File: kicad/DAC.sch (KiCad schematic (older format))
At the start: 27 parts, among them Q1 Q_DUAL_NMOS_S1G1D2S2G2D1, U6 TCR2EE48, U7 DS3911, U8 TSV994IPT

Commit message: 0603 most passives
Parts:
- R11, R12, R13, R14, R15, R16, R17, R18, R19, R20: footprint Resistor_SMD:R_0805_2012Metric_Pad1.20x1.40mm_HandSolder -> Resistor_SMD:R_0603_1608Metric_Pad0.98x0.95mm_HandSolder
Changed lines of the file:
@@
 F 0 "R13" V 8250 3100 50  0000 L CNN
 F 1 "1k" V 8350 3100 50  0000 L CNN
-F 2 "Resistor_SMD:R_0805_2012Metric_Pad1.20x1.40mm_HandSolder" V 8280 3150 50  0001 C CNN
+F 2 "Resistor_SMD:R_0603_1608Metric_Pad0.98x0.95mm_HandSolder" V 8280 3150 50  0001 C CNN
 F 3 "~" H 8350 3150 50  0001 C CNN
 	1    8350 3150
@@
 F 0 "R17" V 8550 3100 50  0000 L CNN
 F 1 "1k" V 8650 3100 50  0000 L CNN
-F 2 "Resistor_SMD:R_0805_2012Metric_Pad1.20x1.40mm_HandSolder" V 8580 3150 50  0001 C CNN
+F 2 "Resistor_SMD:R_0603_1608Metric_Pad0.98x0.95mm_HandSolder" V 8580 3150 50  0001 C CNN
 F 3 "~" H 8650 3150 50  0001 C CNN
 	1    8650 3150
@@
 F 0 "R14" V 8250 3550 50  0000 L CNN
 F 1 "1k" V 8350 3550 50  0000 L CNN
-F 2 "Resistor_SMD:R_0805_2012Metric_Pad1.20x1.40mm_HandSolder" V 8280 3600 50  0001 C CNN
+F 2 "Resistor_SMD:R_0603_1608Metric_Pad0.98x0.95mm_HandSolder" V 8280 3600 50  0001 C CNN
 F 3 "~" H 8350 3600 50  0001 C CNN
 	1    8350 3600
@@
 F 0 "R18" V 8550 3550 50  0000 L CNN
 F 1 "1k" V 8650 3550 50  0000 L CNN
-F 2 "Resistor_SMD:R_0805_2012Metric_Pad1.20x1.40mm_HandSolder" V 8580 3600 50  0001 C CNN
+F 2 "Resistor_SMD:R_0603_1608Metric_Pad0.98x0.95mm_HandSolder" V 8580 3600 50  0001 C CNN
 F 3 "~" H 8650 3600 50  0001 C CNN
 	1    8650 3600
@@
 F 0 "R15" V 8250 4050 50  0000 L CNN
 F 1 "1k" V 8350 4050 50  0000 L CNN
-F 2 "Resistor_SMD:R_0805_2012Metric_Pad1.20x1.40mm_HandSolder" V 8280 4100 50  0001 C CNN
+F 2 "Resistor_SMD:R_0603_1608Metric_Pad0.98x0.95mm_HandSolder" V 8280 4100 50  0001 C CNN
 F 3 "~" H 8350 4100 50  0001 C CNN
 	1    8350 4100
@@
 F 0 "R19" V 8550 4050 50  0000 L CNN
 F 1 "1k" V 8650 4050 50  0000 L CNN
-F 2 "Resistor_SMD:R_0805_2012Metric_Pad1.20x1.40mm_HandSolder" V 8580 4100 50  0001 C CNN
+F 2 "Resistor_SMD:R_0603_1608Metric_Pad0.98x0.95mm_HandSolder" V 8580 4100 50  0001 C CNN
 F 3 "~" H 8650 4100 50  0001 C CNN
 	1    8650 4100
@@
 F 0 "R16" V 8250 4550 50  0000 L CNN
 F 1 "1k" V 8350 4550 50  0000 L CNN
-F 2 "Resistor_SMD:R_0805_2012Metric_Pad1.20x1.40mm_HandSolder" V 8280 4600 50  0001 C CNN
+F 2 "Resistor_SMD:R_0603_1608Metric_Pad0.98x0.95mm_HandSolder" V 8280 4600 50  0001 C CNN
 F 3 "~" H 8350 4600 50  0001 C CNN
 	1    8350 4600
@@
 F 0 "R20" V 8550 4550 50  0000 L CNN
 F 1 "1k" V 8650 4550 50  0000 L CNN
-F 2 "Resistor_SMD:R_0805_2012Metric_Pad1.20x1.40mm_HandSolder" V 8580 4600 50  0001 C CNN
+F 2 "Resistor_SMD:R_0603_1608Metric_Pad0.98x0.95mm_HandSolder" V 8580 4600 50  0001 C CNN
 F 3 "~" H 8650 4600 50  0001 C CNN
 	1    8650 4600
@@
 F 0 "R11" H 4170 5396 50  0000 L CNN
 F 1 "4.7k" H 4170 5305 50  0000 L CNN
-F 2 "Resistor_SMD:R_0805_2012Metric_Pad1.20x1.40mm_HandSolder" V 4030 5350 50  0001 C CNN
+F 2 "Resistor_SMD:R_0603_1608Metric_Pad0.98x0.95mm_HandSolder" V 4030 5350 50  0001 C CNN
 F 3 "~" H 4100 5350 50  0001 C CNN
 	1    4100 5350
@@
 F 0 "R12" H 4470 5396 50  0000 L CNN
 F 1 "4.7k" H 4470 5305 50  0000 L CNN
-F 2 "Resistor_SMD:R_0805_2012Metric_Pad1.20x1.40mm_HandSolder" V 4330 5350 50  0001 C CNN
+F 2 "Resistor_SMD:R_0603_1608Metric_Pad0.98x0.95mm_HandSolder" V 4330 5350 50  0001 C CNN
 F 3 "~" H 4400 5350 50  0001 C CNN
 	1    4400 5350

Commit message: adding jlc fields
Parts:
- C12, C14, C15, C16, C17, C18, C19, C20, C21, C22, C23: JLC (none) -> 0603; LCSC (none) -> C30926
- C13, C24: JLC (none) -> 0805; LCSC (none) -> C215803
- U6: JLC (none) -> SOT-23-5; LCSC (none) -> C698019
- U7: JLC (none) -> TDFN-14-EP(3x3); LCSC (none) -> C1554592
- U8: JLC (none) -> TSSOP-14; LCSC (none) -> C503311
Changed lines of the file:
@@
 F 2 "quadrant:SON40P300X500X80-15N" H 7900 3600 50  0001 C CNN
 F 3 "" H 7900 3600 50  0001 C CNN
+F 4 "TDFN-14-EP(3x3)" H 7900 3600 50  0001 C CNN "JLC"
+F 5 "C1554592" H 7900 3600 50  0001 C CNN "LCSC"
 	1    7900 3600
 	1    0    0    -1
@@
 F 2 "Capacitor_SMD:C_0603_1608Metric_Pad1.08x0.95mm_HandSolder" H 7150 3200 50  0001 C CNN
 F 3 "~" H 7150 3200 50  0001 C CNN
+F 4 "0603" H 7150 3200 50  0001 C CNN "JLC"
+F 5 "C30926" H 7150 3200 50  0001 C CNN "LCSC"
 	1    7150 3200
 	1    0    0    -1
@@
 F 2 "Capacitor_SMD:C_0603_1608Metric_Pad1.08x0.95mm_HandSolder" H 7150 3600 50  0001 C CNN
 F 3 "~" H 7150 3600 50  0001 C CNN
+F 4 "0603" H 7150 3600 50  0001 C CNN "JLC"
+F 5 "C30926" H 7150 3600 50  0001 C CNN "LCSC"
 	1    7150 3600
 	1    0    0    -1
@@
 F 2 "Capacitor_SMD:C_0603_1608Metric_Pad1.08x0.95mm_HandSolder" H 8500 3250 50  0001 C CNN
 F 3 "~" H 8500 3250 50  0001 C CNN
+F 4 "0603" H 8500 3250 50  0001 C CNN "JLC"
+F 5 "C30926" H 8500 3250 50  0001 C CNN "LCSC"
 	1    8500 3250
 	-1   0    0    1
@@
 F 2 "Capacitor_SMD:C_0603_1608Metric_Pad1.08x0.95mm_HandSolder" H 8800 3250 50  0001 C CNN
 F 3 "~" H 8800 3250 50  0001 C CNN
+F 4 "0603" H 8800 3250 50  0001 C CNN "JLC"
+F 5 "C30926" H 8800 3250 50  0001 C CNN "LCSC"
 	1    8800 3250
 	-1   0    0    1
@@
 F 2 "Capacitor_SMD:C_0603_1608Metric_Pad1.08x0.95mm_HandSolder" H 8500 3700 50  0001 C CNN
 F 3 "~" H 8500 3700 50  0001 C CNN
+F 4 "0603" H 8500 3700 50  0001 C CNN "JLC"
+F 5 "C30926" H 8500 3700 50  0001 C CNN "LCSC"
 	1    8500 3700
 	-1   0    0    1
@@
 F 2 "Capacitor_SMD:C_0603_1608Metric_Pad1.08x0.95mm_HandSolder" H 8800 3700 50  0001 C CNN
 F 3 "~" H 8800 3700 50  0001 C CNN
+F 4 "0603" H 8800 3700 50  0001 C CNN "JLC"
+F 5 "C30926" H 8800 3700 50  0001 C CNN "LCSC"
 	1    8800 3700
 	-1   0    0    1
@@
 F 2 "Capacitor_SMD:C_0603_1608Metric_Pad1.08x0.95mm_HandSolder" H 8500 4200 50  0001 C CNN
 F 3 "~" H 8500 4200 50  0001 C CNN
+F 4 "0603" H 8500 4200 50  0001 C CNN "JLC"
+F 5 "C30926" H 8500 4200 50  0001 C CNN "LCSC"
 	1    8500 4200
 	-1   0    0    1
@@
 F 2 "Capacitor_SMD:C_0603_1608Metric_Pad1.08x0.95mm_HandSolder" H 8800 4200 50  0001 C CNN
 F 3 "~" H 8800 4200 50  0001 C CNN
+F 4 "0603" H 8800 4200 50  0001 C CNN "JLC"
+F 5 "C30926" H 8800 4200 50  0001 C CNN "LCSC"
 	1    8800 4200
 	-1   0    0    1
@@
 F 2 "Capacitor_SMD:C_0603_1608Metric_Pad1.08x0.95mm_HandSolder" H 8800 4700 50  0001 C CNN
 F 3 "~" H 8800 4700 50  0001 C CNN
+F 4 "0603" H 8800 4700 50  0001 C CNN "JLC"
+F 5 "C30926" H 8800 4700 50  0001 C CNN "LCSC"
 	1    8800 4700
 	-1   0    0    1
@@
 F 2 "Package_SO:TSSOP-14_4.4x5mm_P0.65mm" H 9450 4200 50  0001 C CNN
 F 3 "~" H 9450 4200 50  0001 C CNN
+F 4 "TSSOP-14" H 9450 4200 50  0001 C CNN "JLC"
+F 5 "C503311" H 9450 4200 50  0001 C CNN "LCSC"
 	1    9450 4200
 	1    0    0    -1
@@
 F 2 "Package_SO:TSSOP-14_4.4x5mm_P0.65mm" H 9450 4700 50  0001 C CNN
 F 3 "~" H 9450 4700 50  0001 C CNN
+F 4 "TSSOP-14" H 9450 4700 50  0001 C CNN "JLC"
+F 5 "C503311" H 9450 4700 50  0001 C CNN "LCSC"
 	2    9450 4700
 	1    0    0    -1
@@
 F 2 "Package_SO:TSSOP-14_4.4x5mm_P0.65mm" H 9450 3700 50  0001 C CNN
 F 3 "~" H 9450 3700 50  0001 C CNN
+F 4 "TSSOP-14" H 9450 3700 50  0001 C CNN "JLC"
+F 5 "C503311" H 9450 3700 50  0001 C CNN "LCSC"
 	3    9450 3700
 	1    0    0    -1
@@
 F 2 "Package_SO:TSSOP-14_4.4x5mm_P0.65mm" H 9450 3250 50  0001 C CNN
 F 3 "~" H 9450 3250 50  0001 C CNN
+F 4 "TSSOP-14" H 9450 3250 50  0001 C CNN "JLC"
+F 5 "C503311" H 9450 3250 50  0001 C CNN "LCSC"
 	4    9450 3250
 	1    0    0    -1
@@
 F 2 "Package_SO:TSSOP-14_4.4x5mm_P0.65mm" H 9750 5350 50  0001 C CNN
 F 3 "~" H 9750 5350 50  0001 C CNN
+F 4 "TSSOP-14" H 9750 5350 50  0001 C CNN "JLC"
+F 5 "C503311" H 9750 5350 50  0001 C CNN "LCSC"
 	5    9750 5350
 	1    0    0    -1
@@
 F 2 "Capacitor_SMD:C_0805_2012Metric_Pad1.18x1.45mm_HandSolder" H 9388 5200 50  0001 C CNN
 F 3 "~" H 9350 5350 50  0001 C CNN
+F 4 "0805" H 9350 5350 50  0001 C CNN "JLC"
+F 5 "C215803" H 9350 5350 50  0001 C CNN "LCSC"
 	1    9350 5350
 	1    0    0    -1
@@
 F 3 "" H 4550 3550 50  0001 C CNN
 F 4 "https://www.digikey.com/en/products/detail/toshiba-semiconductor-and-storage/TCR2EE48-LM/5114341" H 4550 3550 50  0001 C CNN "digikey"
+F 5 "SOT-23-5" H 4550 3550 50  0001 C CNN "JLC"
+F 6 "C698019" H 4550 3550 50  0001 C CNN "LCSC"
 	1    4550 3550
 	1    0    0    -1
@@
 F 2 "Capacitor_SMD:C_0603_1608Metric_Pad1.08x0.95mm_HandSolder" H 3900 3600 50  0001 C CNN
 F 3 "~" H 3900 3600 50  0001 C CNN
+F 4 "0603" H 3900 3600 50  0001 C CNN "JLC"
+F 5 "C30926" H 3900 3600 50  0001 C CNN "LCSC"
 	1    3900 3600
 	1    0    0    -1
@@
 F 2 "Capacitor_SMD:C_0805_2012Metric_Pad1.18x1.45mm_HandSolder" H 5100 3600 50  0001 C CNN
 F 3 "~" H 5100 3600 50  0001 C CNN
+F 4 "0805" H 5100 3600 50  0001 C CNN "JLC"
+F 5 "C215803" H 5100 3600 50  0001 C CNN "LCSC"
 	1    5100 3600
 	1    0    0    -1
@@
 F 2 "Capacitor_SMD:C_0603_1608Metric_Pad1.08x0.95mm_HandSolder" H 8500 4700 50  0001 C CNN
 F 3 "~" H 8500 4700 50  0001 C CNN
+F 4 "0603" H 8500 4700 50  0001 C CNN "JLC"
+F 5 "C30926" H 8500 4700 50  0001 C CNN "LCSC"
 	1    8500 4700
 	-1   0    0    1

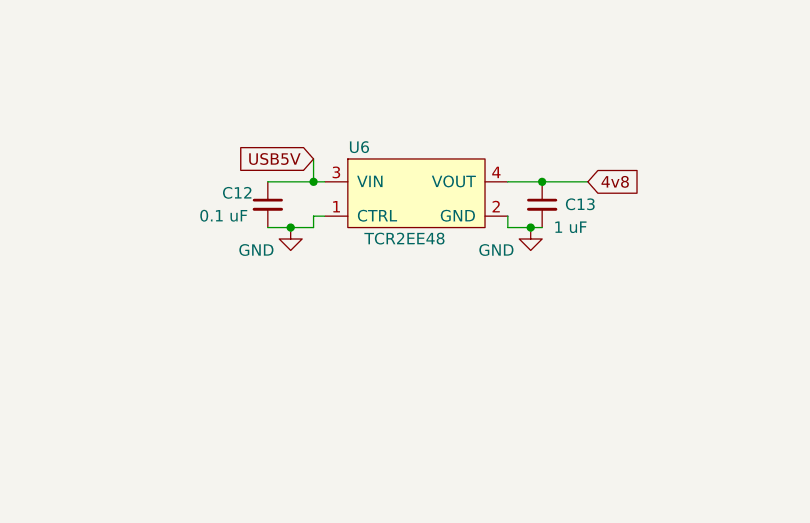
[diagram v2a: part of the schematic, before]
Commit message: more jlc fields
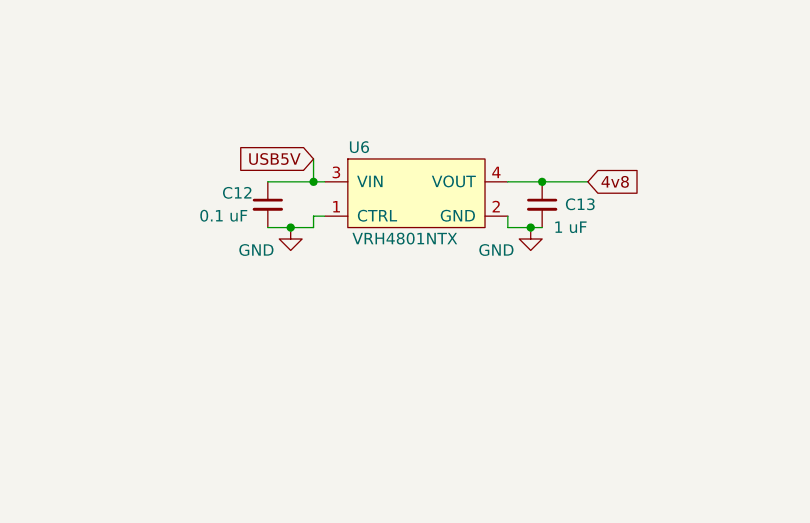
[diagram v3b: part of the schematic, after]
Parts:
- C12, C13, C14, C15, C16, C17, C18, C19, C20, C21, C22, C23, C24, U7, U8: ordered (none) -> y
- R11, R12: JLC (none) -> 0603; LCSC (none) -> C23162; ordered (none) -> y
- R13, R14, R15, R16, R17, R18, R19, R20: JLC (none) -> 0603; LCSC (none) -> C21190; ordered (none) -> y
- U6: value TCR2EE48 -> VRH4801NTX; ordered (none) -> ---
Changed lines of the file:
@@
 F 4 "TDFN-14-EP(3x3)" H 7900 3600 50  0001 C CNN "JLC"
 F 5 "C1554592" H 7900 3600 50  0001 C CNN "LCSC"
+F 6 "y" H 7900 3600 50  0001 C CNN "ordered"
 	1    7900 3600
 	1    0    0    -1
@@
 F 4 "0603" H 7150 3200 50  0001 C CNN "JLC"
 F 5 "C30926" H 7150 3200 50  0001 C CNN "LCSC"
+F 6 "y" H 7150 3200 50  0001 C CNN "ordered"
 	1    7150 3200
 	1    0    0    -1
@@
 F 4 "0603" H 7150 3600 50  0001 C CNN "JLC"
 F 5 "C30926" H 7150 3600 50  0001 C CNN "LCSC"
+F 6 "y" H 7150 3600 50  0001 C CNN "ordered"
 	1    7150 3600
 	1    0    0    -1
@@
 F 2 "Resistor_SMD:R_0603_1608Metric_Pad0.98x0.95mm_HandSolder" V 8280 3150 50  0001 C CNN
 F 3 "~" H 8350 3150 50  0001 C CNN
+F 4 "0603" H 8350 3150 50  0001 C CNN "JLC"
+F 5 " C21190 " H 8350 3150 50  0001 C CNN "LCSC"
+F 6 "y" H 8350 3150 50  0001 C CNN "ordered"
 	1    8350 3150
 	0    -1   1    0
@@
 F 4 "0603" H 8500 3250 50  0001 C CNN "JLC"
 F 5 "C30926" H 8500 3250 50  0001 C CNN "LCSC"
+F 6 "y" H 8500 3250 50  0001 C CNN "ordered"
 	1    8500 3250
 	-1   0    0    1
@@
 F 4 "0603" H 8800 3250 50  0001 C CNN "JLC"
 F 5 "C30926" H 8800 3250 50  0001 C CNN "LCSC"
+F 6 "y" H 8800 3250 50  0001 C CNN "ordered"
 	1    8800 3250
 	-1   0    0    1
@@
 F 2 "Resistor_SMD:R_0603_1608Metric_Pad0.98x0.95mm_HandSolder" V 8580 3150 50  0001 C CNN
 F 3 "~" H 8650 3150 50  0001 C CNN
+F 4 "0603" H 8650 3150 50  0001 C CNN "JLC"
+F 5 " C21190 " H 8650 3150 50  0001 C CNN "LCSC"
+F 6 "y" H 8650 3150 50  0001 C CNN "ordered"
 	1    8650 3150
 	0    -1   1    0
@@
 F 2 "Resistor_SMD:R_0603_1608Metric_Pad0.98x0.95mm_HandSolder" V 8280 3600 50  0001 C CNN
 F 3 "~" H 8350 3600 50  0001 C CNN
+F 4 "0603" H 8350 3600 50  0001 C CNN "JLC"
+F 5 " C21190 " H 8350 3600 50  0001 C CNN "LCSC"
+F 6 "y" H 8350 3600 50  0001 C CNN "ordered"
 	1    8350 3600
 	0    -1   1    0
@@
 F 4 "0603" H 8500 3700 50  0001 C CNN "JLC"
 F 5 "C30926" H 8500 3700 50  0001 C CNN "LCSC"
+F 6 "y" H 8500 3700 50  0001 C CNN "ordered"
 	1    8500 3700
 	-1   0    0    1
@@
 F 4 "0603" H 8800 3700 50  0001 C CNN "JLC"
 F 5 "C30926" H 8800 3700 50  0001 C CNN "LCSC"
+F 6 "y" H 8800 3700 50  0001 C CNN "ordered"
 	1    8800 3700
 	-1   0    0    1
@@
 F 2 "Resistor_SMD:R_0603_1608Metric_Pad0.98x0.95mm_HandSolder" V 8580 3600 50  0001 C CNN
 F 3 "~" H 8650 3600 50  0001 C CNN
+F 4 "0603" H 8650 3600 50  0001 C CNN "JLC"
+F 5 " C21190 " H 8650 3600 50  0001 C CNN "LCSC"
+F 6 "y" H 8650 3600 50  0001 C CNN "ordered"
 	1    8650 3600
 	0    -1   1    0
@@
 F 2 "Resistor_SMD:R_0603_1608Metric_Pad0.98x0.95mm_HandSolder" V 8280 4100 50  0001 C CNN
 F 3 "~" H 8350 4100 50  0001 C CNN
+F 4 "0603" H 8350 4100 50  0001 C CNN "JLC"
+F 5 " C21190 " H 8350 4100 50  0001 C CNN "LCSC"
+F 6 "y" H 8350 4100 50  0001 C CNN "ordered"
 	1    8350 4100
 	0    -1   1    0
@@
 F 4 "0603" H 8500 4200 50  0001 C CNN "JLC"
 F 5 "C30926" H 8500 4200 50  0001 C CNN "LCSC"
+F 6 "y" H 8500 4200 50  0001 C CNN "ordered"
 	1    8500 4200
 	-1   0    0    1
@@
 F 4 "0603" H 8800 4200 50  0001 C CNN "JLC"
 F 5 "C30926" H 8800 4200 50  0001 C CNN "LCSC"
+F 6 "y" H 8800 4200 50  0001 C CNN "ordered"
 	1    8800 4200
 	-1   0    0    1
@@
 F 2 "Resistor_SMD:R_0603_1608Metric_Pad0.98x0.95mm_HandSolder" V 8580 4100 50  0001 C CNN
 F 3 "~" H 8650 4100 50  0001 C CNN
+F 4 "0603" H 8650 4100 50  0001 C CNN "JLC"
+F 5 " C21190 " H 8650 4100 50  0001 C CNN "LCSC"
+F 6 "y" H 8650 4100 50  0001 C CNN "ordered"
 	1    8650 4100
 	0    -1   1    0
@@
 F 2 "Resistor_SMD:R_0603_1608Metric_Pad0.98x0.95mm_HandSolder" V 8280 4600 50  0001 C CNN
 F 3 "~" H 8350 4600 50  0001 C CNN
+F 4 "0603" H 8350 4600 50  0001 C CNN "JLC"
+F 5 " C21190 " H 8350 4600 50  0001 C CNN "LCSC"
+F 6 "y" H 8350 4600 50  0001 C CNN "ordered"
 	1    8350 4600
 	0    -1   1    0
@@
 F 4 "0603" H 8800 4700 50  0001 C CNN "JLC"
 F 5 "C30926" H 8800 4700 50  0001 C CNN "LCSC"
+F 6 "y" H 8800 4700 50  0001 C CNN "ordered"
 	1    8800 4700
 	-1   0    0    1
@@
 F 2 "Resistor_SMD:R_0603_1608Metric_Pad0.98x0.95mm_HandSolder" V 8580 4600 50  0001 C CNN
 F 3 "~" H 8650 4600 50  0001 C CNN
+F 4 "0603" H 8650 4600 50  0001 C CNN "JLC"
+F 5 " C21190 " H 8650 4600 50  0001 C CNN "LCSC"
+F 6 "y" H 8650 4600 50  0001 C CNN "ordered"
 	1    8650 4600
 	0    -1   1    0
@@
 F 4 "TSSOP-14" H 9450 4200 50  0001 C CNN "JLC"
 F 5 "C503311" H 9450 4200 50  0001 C CNN "LCSC"
+F 6 "y" H 9450 4200 50  0001 C CNN "ordered"
 	1    9450 4200
 	1    0    0    -1
@@
 F 4 "TSSOP-14" H 9450 4700 50  0001 C CNN "JLC"
 F 5 "C503311" H 9450 4700 50  0001 C CNN "LCSC"
+F 6 "y" H 9450 4700 50  0001 C CNN "ordered"
 	2    9450 4700
 	1    0    0    -1
@@
 F 4 "TSSOP-14" H 9450 3700 50  0001 C CNN "JLC"
 F 5 "C503311" H 9450 3700 50  0001 C CNN "LCSC"
+F 6 "y" H 9450 3700 50  0001 C CNN "ordered"
 	3    9450 3700
 	1    0    0    -1
@@
 F 4 "TSSOP-14" H 9450 3250 50  0001 C CNN "JLC"
 F 5 "C503311" H 9450 3250 50  0001 C CNN "LCSC"
+F 6 "y" H 9450 3250 50  0001 C CNN "ordered"
 	4    9450 3250
 	1    0    0    -1
@@
 F 4 "TSSOP-14" H 9750 5350 50  0001 C CNN "JLC"
 F 5 "C503311" H 9750 5350 50  0001 C CNN "LCSC"
+F 6 "y" H 9750 5350 50  0001 C CNN "ordered"
 	5    9750 5350
 	1    0    0    -1
@@
 F 4 "0805" H 9350 5350 50  0001 C CNN "JLC"
 F 5 "C215803" H 9350 5350 50  0001 C CNN "LCSC"
+F 6 "y" H 9350 5350 50  0001 C CNN "ordered"
 	1    9350 5350
 	1    0    0    -1
@@
 F 2 "Resistor_SMD:R_0603_1608Metric_Pad0.98x0.95mm_HandSolder" V 4030 5350 50  0001 C CNN
 F 3 "~" H 4100 5350 50  0001 C CNN
+F 4 "0603" H 4100 5350 50  0001 C CNN "JLC"
+F 5 " C23162 " H 4100 5350 50  0001 C CNN "LCSC"
+F 6 "y" H 4100 5350 50  0001 C CNN "ordered"
 	1    4100 5350
 	-1   0    0    -1
@@
 F 2 "Resistor_SMD:R_0603_1608Metric_Pad0.98x0.95mm_HandSolder" V 4330 5350 50  0001 C CNN
 F 3 "~" H 4400 5350 50  0001 C CNN
+F 4 "0603" H 4400 5350 50  0001 C CNN "JLC"
+F 5 " C23162 " H 4400 5350 50  0001 C CNN "LCSC"
+F 6 "y" H 4400 5350 50  0001 C CNN "ordered"
 	1    4400 5350
 	-1   0    0    -1
@@
 AR Path="/63922B28/63AF8548" Ref="U6"  Part="1"
 F 0 "U6" H 4300 3750 50  0000 C CNN
-F 1 "TCR2EE48" H 4500 3350 50  0000 C CNN
+F 1 "VRH4801NTX" H 4500 3350 50  0000 C CNN
 F 2 "Package_TO_SOT_SMD:SOT-553" H 4550 3550 50  0001 C CNN
 F 3 "" H 4550 3550 50  0001 C CNN
@@
 F 5 "SOT-23-5" H 4550 3550 50  0001 C CNN "JLC"
 F 6 "C698019" H 4550 3550 50  0001 C CNN "LCSC"
+F 7 "---" H 4550 3550 50  0001 C CNN "ordered"
 	1    4550 3550
 	1    0    0    -1
@@
 F 4 "0603" H 3900 3600 50  0001 C CNN "JLC"
 F 5 "C30926" H 3900 3600 50  0001 C CNN "LCSC"
+F 6 "y" H 3900 3600 50  0001 C CNN "ordered"
 	1    3900 3600
 	1    0    0    -1
@@
 F 4 "0805" H 5100 3600 50  0001 C CNN "JLC"
 F 5 "C215803" H 5100 3600 50  0001 C CNN "LCSC"
+F 6 "y" H 5100 3600 50  0001 C CNN "ordered"
 	1    5100 3600
 	1    0    0    -1
@@
 F 4 "0603" H 8500 4700 50  0001 C CNN "JLC"
 F 5 "C30926" H 8500 4700 50  0001 C CNN "LCSC"
+F 6 "y" H 8500 4700 50  0001 C CNN "ordered"
 	1    8500 4700
 	-1   0    0    1
